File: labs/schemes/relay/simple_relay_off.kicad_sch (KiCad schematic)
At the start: 3 parts, among them SW2 Операнд 2

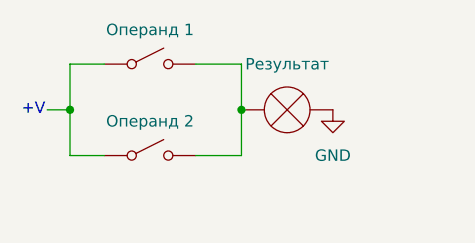
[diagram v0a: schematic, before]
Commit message: Many updates
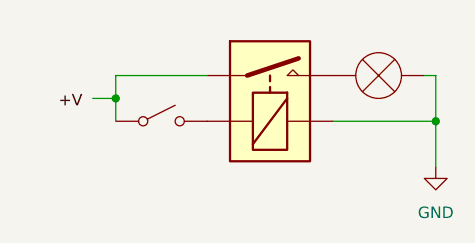
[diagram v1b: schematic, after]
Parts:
- removed LA2: Результат, symbol Device:Lamp
- removed SW2: Операнд 2, symbol Switch:SW_DPST_x2
- removed Операнд11: Операнд 1, symbol Switch:SW_DPST_x2
- added K4: 4PDT, relay:MY4N socket, symbol relay:4PDT
- added LA?: Lamp, symbol Device:Lamp
- added SW?: SW_DPST_x2, symbol Switch:SW_DPST_x2
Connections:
- net GND: now also K4.13, LA?.1 (-)
- new net: K4.12, SW?.1 (A)
- new net: K4.14, SW?.2 (B)
- new net: K4.8, LA?.2 (+)
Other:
- note removed: "+V"
